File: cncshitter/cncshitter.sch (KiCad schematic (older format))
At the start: 71 parts, among them J1 24V_IN, J2 5V_IN, J3 DB25_Male_MountingHoles, J4 Screw_Terminal_01x11, J5 Screw_Terminal_01x06, K1 SANYOU_SRD_Form_C, K2 SANYOU_SRD_Form_C, Q1 BC847, Q2 BC847, Q3 BC847, Q4 BC847, Q5 BC847, Q6 BC847, Q7 BC847, Q8 BC847, Q9 BC847, U1 EMERGENCY, U10 AXIS_Y_STEP, U11 AXIS_Z_DIR, U12 AXIS_Z_STEP, U2 PROBE, U3 ENABLE, U4 SPINDLE_PWM, U5 SPINDLE_ENC, U6 SPINDLE_ENABLE, U7 AXIS_X_DIR, U8 AXIS_X_STEP, U9 AXIS_Y_DIR

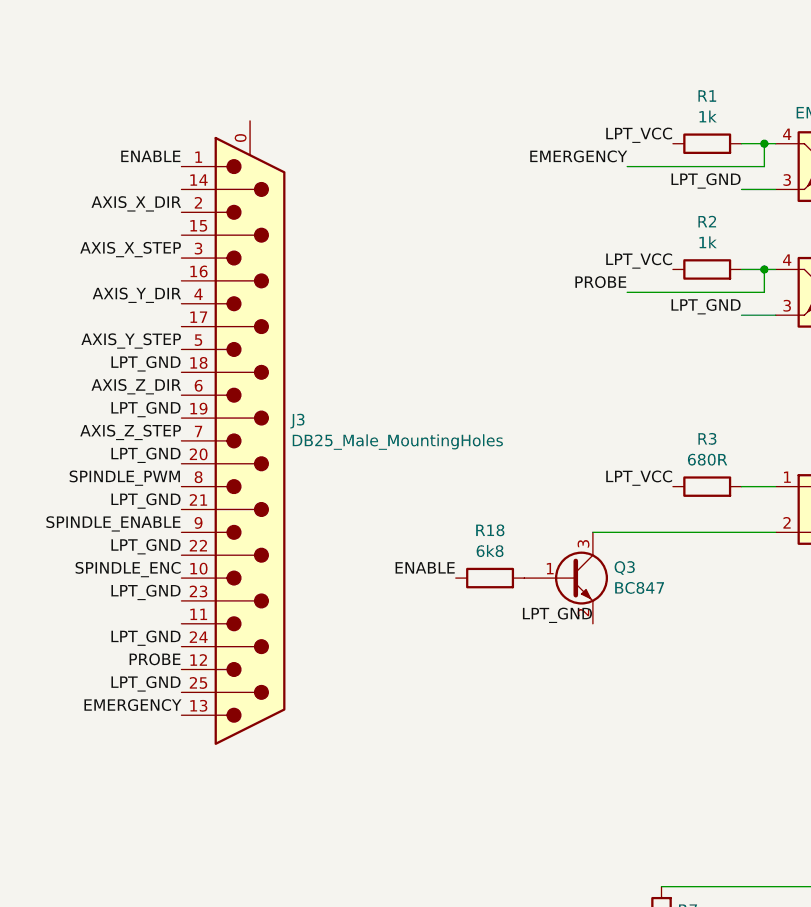
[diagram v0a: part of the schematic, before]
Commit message: vkkt
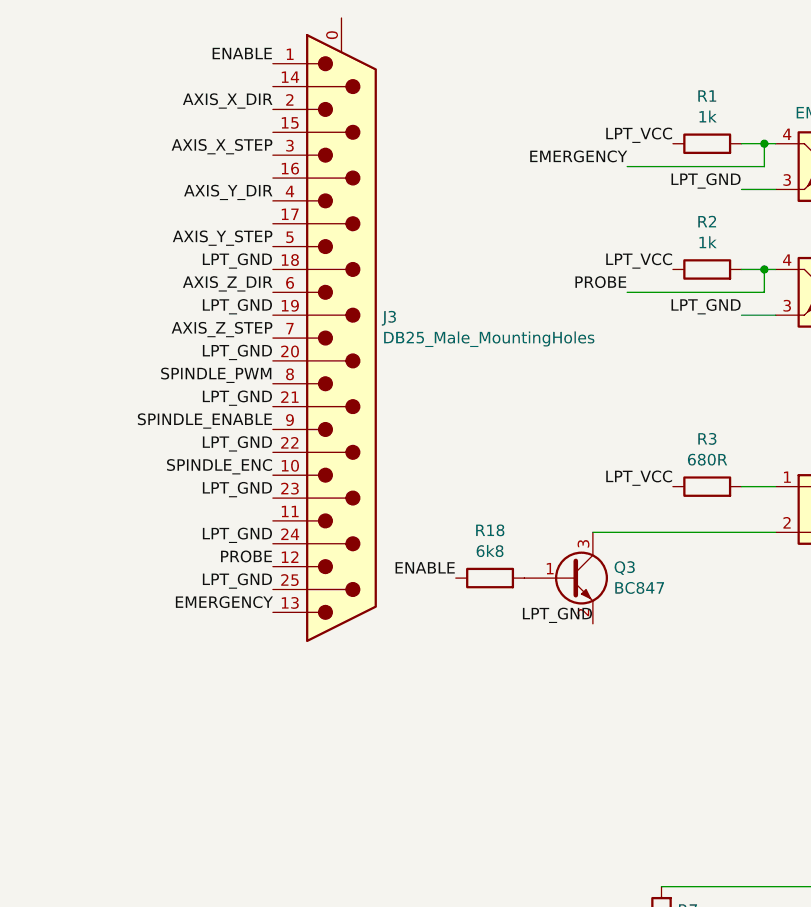
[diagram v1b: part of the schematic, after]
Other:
- moved on the sheet: J3
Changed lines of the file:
@@
 L Connector:DB25_Male_MountingHoles J3
 U 1 1 5E18E720
-P 1500 2600
-F 0 "J3" H 1680 2509 50  0000 L CNN
-F 1 "DB25_Male_MountingHoles" H 1680 2600 50  0000 L CNN
-F 2 "Connector_Dsub:DSUB-25_Male_Horizontal_P2.77x2.84mm_EdgePinOffset7.70mm_Housed_MountingHolesOffset9.12mm" H 1500 2600 50  0001 C CNN
-F 3 " ~" H 1500 2600 50  0001 C CNN
-	1    1500 2600
+P 1900 2150
+F 0 "J3" H 2080 2059 50  0000 L CNN
+F 1 "DB25_Male_MountingHoles" H 2080 2150 50  0000 L CNN
+F 2 "Connector_Dsub:DSUB-25_Male_Horizontal_P2.77x2.84mm_EdgePinOffset7.70mm_Housed_MountingHolesOffset9.12mm" H 1900 2150 50  0001 C CNN
+F 3 " ~" H 1900 2150 50  0001 C CNN
+	1    1900 2150
 	1    0    0    1
 $EndComp
@@
 Text Label 6350 6100 0    50   ~ 0
 LPT_VCC
-Text Label 1200 3700 2    50   ~ 0
-LPT_GND
-Text Label 1200 3500 2    50   ~ 0
-LPT_GND
-Text Label 1200 3300 2    50   ~ 0
-LPT_GND
-Text Label 1200 3100 2    50   ~ 0
-LPT_GND
-Text Label 1200 2900 2    50   ~ 0
-LPT_GND
-Text Label 1200 2700 2    50   ~ 0
-LPT_GND
-Text Label 1200 2500 2    50   ~ 0
-LPT_GND
-Text Label 1200 2300 2    50   ~ 0
-LPT_GND
-Text Label 1200 1600 2    50   ~ 0
+Text Label 1600 3250 2    50   ~ 0
+LPT_GND
+Text Label 1600 3050 2    50   ~ 0
+LPT_GND
+Text Label 1600 2850 2    50   ~ 0
+LPT_GND
+Text Label 1600 2650 2    50   ~ 0
+LPT_GND
+Text Label 1600 2450 2    50   ~ 0
+LPT_GND
+Text Label 1600 2250 2    50   ~ 0
+LPT_GND
+Text Label 1600 2050 2    50   ~ 0
+LPT_GND
+Text Label 1600 1850 2    50   ~ 0
+LPT_GND
+Text Label 1600 1150 2    50   ~ 0
 AXIS_X_DIR
-Text Label 1200 1800 2    50   ~ 0
+Text Label 1600 1350 2    50   ~ 0
 AXIS_X_STEP
-Text Label 1200 2000 2    50   ~ 0
+Text Label 1600 1550 2    50   ~ 0
 AXIS_Y_DIR
-Text Label 1200 2200 2    50   ~ 0
+Text Label 1600 1750 2    50   ~ 0
 AXIS_Y_STEP
-Text Label 1200 2400 2    50   ~ 0
+Text Label 1600 1950 2    50   ~ 0
 AXIS_Z_DIR
-Text Label 1200 2600 2    50   ~ 0
+Text Label 1600 2150 2    50   ~ 0
 AXIS_Z_STEP
-Text Label 1200 1400 2    50   ~ 0
+Text Label 1600 950  2    50   ~ 0
 ENABLE
-Text Label 1200 3600 2    50   ~ 0
+Text Label 1600 3150 2    50   ~ 0
 PROBE
-Text Label 1200 3800 2    50   ~ 0
+Text Label 1600 3350 2    50   ~ 0
 EMERGENCY
-Text Label 1200 3200 2    50   ~ 0
+Text Label 1600 2750 2    50   ~ 0
 SPINDLE_ENC
-Text Label 1200 2800 2    50   ~ 0
+Text Label 1600 2350 2    50   ~ 0
 SPINDLE_PWM
-Text Label 1200 3000 2    50   ~ 0
+Text Label 1600 2550 2    50   ~ 0
 SPINDLE_ENABLE
 $Comp
